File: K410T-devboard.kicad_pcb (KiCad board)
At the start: 2 copper layers, 120 x 120 mm, 31 parts, among them U1 XC7K410T-2FFG900I, U2 MT41K512M8DA

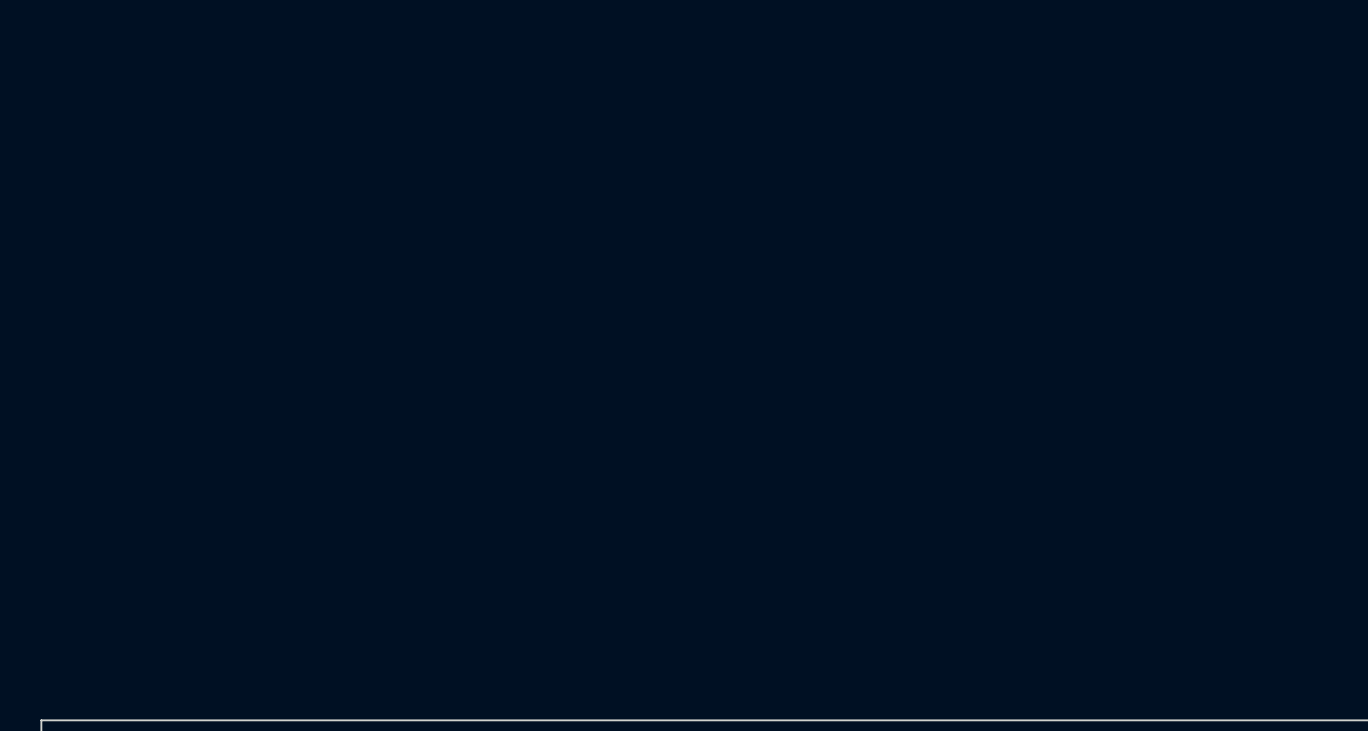
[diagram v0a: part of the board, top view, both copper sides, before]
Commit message: Update project files naming, reorganize hierarchical sheet structure, power supply WIP
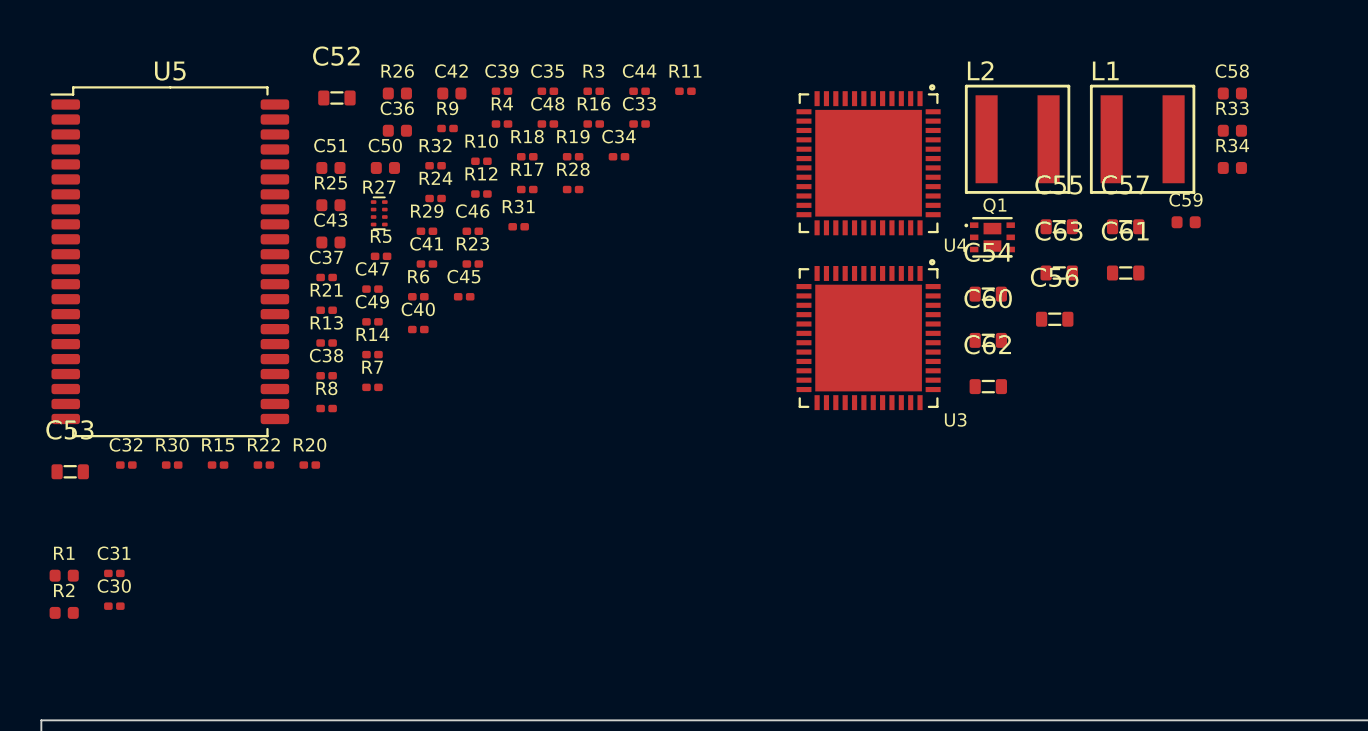
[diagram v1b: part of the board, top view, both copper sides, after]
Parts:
- added C30: C_100n_0201, antmicro-footprints:0201-res, F.Cu at (153.9, 63.9)
- added C31: C_100n_0201, antmicro-footprints:0201-res, F.Cu at (153.9, 62.1)
- added C32: C_100n_0201, antmicro-footprints:0201-res, F.Cu at (154.5, 56.4)
- added C33: C_100n_0201, antmicro-footprints:0201-res, F.Cu at (182.0, 38.1)
- added C34: C_100n_0201, antmicro-footprints:0201-res, F.Cu at (180.9, 39.9)
- added C35: C_100n_0201, antmicro-footprints:0201-res, F.Cu at (177.1, 36.4)
- added C36: C_10u_0402, antmicro-footprints:0402-cap, F.Cu at (169.0, 38.5)
- added C37: C_100n_0201, antmicro-footprints:0201-res, F.Cu at (165.2, 46.3)
- added C38: C_100n_0201, antmicro-footprints:0201-res, F.Cu at (165.2, 51.6)
- added C39: C_100n_0201, antmicro-footprints:0201-res, F.Cu at (174.6, 36.4)
- added C40: C_100n_0201, antmicro-footprints:0201-res, F.Cu at (170.1, 49.1)
- added C41: C_100n_0201, antmicro-footprints:0201-res, F.Cu at (170.6, 45.6)
- added C42: C_10u_0402, antmicro-footprints:0402-cap, F.Cu at (171.9, 36.5)
- added C43: C_10u_0402, antmicro-footprints:0402-cap, F.Cu at (165.5, 44.5)
- added C44: C_100n_0201, antmicro-footprints:0201-res, F.Cu at (182.0, 36.4)
- added C45: C_100n_0201, antmicro-footprints:0201-res, F.Cu at (172.6, 47.4)
- added C46: C_100n_0201, antmicro-footprints:0201-res, F.Cu at (173.1, 43.9)
- added C47: C_100n_0201, antmicro-footprints:0201-res, F.Cu at (167.7, 47.0)
- added C48: C_100n_0201, antmicro-footprints:0201-res, F.Cu at (177.1, 38.1)
- added C49: C_100n_0201, antmicro-footprints:0201-res, F.Cu at (167.7, 48.7)
- added C50: C_4u7_0402, antmicro-footprints:0402-cap, F.Cu at (168.4, 40.5)
- added C51: C_4u7_0402, antmicro-footprints:0402-cap, F.Cu at (165.5, 40.5)
- added C52: C_47u_0603, antmicro-footprints:0603-cap, F.Cu at (165.8, 36.8)
- added C53: C_47u_0603, antmicro-footprints:0603-cap, F.Cu at (151.5, 56.7)
- added C54: C_10u_25V_0603, antmicro-footprints:0603-cap, F.Cu at (200.6, 47.2)
- added C55: C_10u_25V_0603, antmicro-footprints:0603-cap, F.Cu at (204.4, 43.6)
- added C56: C_10u_25V_0603, antmicro-footprints:0603-cap, F.Cu at (204.1, 48.6)
- added C57: C_10u_25V_0603, antmicro-footprints:0603-cap, F.Cu at (207.9, 43.6)
- added C58: C_100n_0402, antmicro-footprints:0402-cap, F.Cu at (213.6, 36.5)
- added C59: C_100n_0402, antmicro-footprints:0402-cap, F.Cu at (211.2, 43.4)
- added C60: C_47u_0603, antmicro-footprints:0603-cap, F.Cu at (200.6, 49.7)
- added C61: C_47u_0603, antmicro-footprints:0603-cap, F.Cu at (207.9, 46.1)
- added C62: C_47u_0603, antmicro-footprints:0603-cap, F.Cu at (200.6, 52.2)
- added C63: C_47u_0603, antmicro-footprints:0603-cap, F.Cu at (204.4, 46.1)
- added L1: XAL5030-122MEC, antmicro-footprints:Coilcraft-XAL5030, F.Cu at (208.8, 39.0)
- added L2: XAL5030-122MEC, antmicro-footprints:Coilcraft-XAL5030, F.Cu at (202.2, 39.0)
- added Q1: SIA906EDJ-T1-GE3, antmicro-footprints:VISHAY_PowerPAK_SC70-6L, F.Cu at (200.8, 44.2)
- added R1: R_80R6_0402, antmicro-footprints:0402-res, F.Cu at (151.2, 62.3)
- added R10: R_40R2_0201, antmicro-footprints:0201-res, F.Cu at (173.5, 40.1)
- added R11: R_40R2_0201, antmicro-footprints:0201-res, F.Cu at (184.4, 36.4)
- added R12: R_40R2_0201, antmicro-footprints:0201-res, F.Cu at (173.5, 41.9)
- added R13: R_40R2_0201, antmicro-footprints:0201-res, F.Cu at (165.2, 49.8)
- added R14: R_40R2_0201, antmicro-footprints:0201-res, F.Cu at (167.7, 50.5)
- added R15: R_40R2_0201, antmicro-footprints:0201-res, F.Cu at (159.4, 56.4)
- added R16: R_40R2_0201, antmicro-footprints:0201-res, F.Cu at (179.5, 38.1)
- added R17: R_40R2_0201, antmicro-footprints:0201-res, F.Cu at (176.0, 41.6)
- added R18: R_40R2_0201, antmicro-footprints:0201-res, F.Cu at (176.0, 39.9)
- added R19: R_40R2_0201, antmicro-footprints:0201-res, F.Cu at (178.4, 39.9)
- added R2: R_80R6_0402, antmicro-footprints:0402-res, F.Cu at (151.2, 64.3)
- added R20: R_40R2_0201, antmicro-footprints:0201-res, F.Cu at (164.3, 56.4)
- added R21: R_40R2_0201, antmicro-footprints:0201-res, F.Cu at (165.2, 48.1)
- added R22: R_40R2_0201, antmicro-footprints:0201-res, F.Cu at (161.9, 56.4)
- added R23: R_100R_0201, antmicro-footprints:0201-res, F.Cu at (173.1, 45.6)
- added R24: R_40R2_0201, antmicro-footprints:0201-res, F.Cu at (171.1, 42.1)
- added R25: R_10k_0402, antmicro-footprints:0402-res, F.Cu at (165.5, 42.5)
- added R26: R_240R_1%_0402, antmicro-footprints:0402-res, F.Cu at (169.0, 36.5)
- added R27: 4x39R_0201_array, antmicro-footprints:EXB18V, F.Cu at (168.1, 42.9)
- added R28: R_40R2_0201, antmicro-footprints:0201-res, F.Cu at (178.4, 41.6)
- added R29: R_40R2_0201, antmicro-footprints:0201-res, F.Cu at (170.6, 43.9)
- added R3: R_40R2_0201, antmicro-footprints:0201-res, F.Cu at (179.5, 36.4)
- added R30: R_40R2_0201, antmicro-footprints:0201-res, F.Cu at (157.0, 56.4)
- added R31: R_40R2_0201, antmicro-footprints:0201-res, F.Cu at (175.5, 43.6)
- added R32: R_40R2_0201, antmicro-footprints:0201-res, F.Cu at (171.1, 40.4)
- added R33: R_22k_0402, antmicro-footprints:0402-res, F.Cu at (213.6, 38.5)
- added R34: R_22k_0402, antmicro-footprints:0402-res, F.Cu at (213.6, 40.5)
- added R4: R_40R2_0201, antmicro-footprints:0201-res, F.Cu at (174.6, 38.1)
- added R5: R_40R2_0201, antmicro-footprints:0201-res, F.Cu at (168.2, 45.2)
- added R6: R_40R2_0201, antmicro-footprints:0201-res, F.Cu at (170.1, 47.4)
- added R7: R_40R2_0201, antmicro-footprints:0201-res, F.Cu at (167.7, 52.2)
- added R8: R_40R2_0201, antmicro-footprints:0201-res, F.Cu at (165.2, 53.3)
- added R9: R_40R2_0201, antmicro-footprints:0201-res, F.Cu at (171.7, 38.4)
- added U3: ADP5054ACPZ-R7, antmicro-footprints:Analog_CP_48_13, F.Cu at (194.2, 49.6)
- added U4: ADP5050ACPZ-R7, antmicro-footprints:Analog_CP_48_13, F.Cu at (194.2, 40.2)
- added U5: AS6C8008-55ZIN, antmicro-footprints:TSOP-II-44_10.16x18.41mm_P0.8mm, F.Cu at (156.9, 45.5)
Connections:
- U1 pad AB7: unconnected-(U1-PadAB7) -> Net-(R2-Pad1)
- U1 pad AC1: unconnected-(U1-PadAC1) -> /FPGA banks 33-34/DDR.A12
- U1 pad AC2: unconnected-(U1-PadAC2) -> /FPGA banks 33-34/DDR.A13
- U1 pad AC4: unconnected-(U1-PadAC4) -> /FPGA banks 33-34/DDR.A10
- U1 pad AC5: unconnected-(U1-PadAC5) -> /FPGA banks 33-34/DDR.A11
- U1 pad AC6: unconnected-(U1-PadAC6) -> /FPGA banks 33-34/DDR_VRN
- U1 pad AC7: unconnected-(U1-PadAC7) -> /FPGA banks 33-34/DDR.A7
- U1 pad AD1: unconnected-(U1-PadAD1) -> /FPGA banks 33-34/DDR.CK_N
- U1 pad AD2: unconnected-(U1-PadAD2) -> /FPGA banks 33-34/DDR.CK_P
- U1 pad AD3: unconnected-(U1-PadAD3) -> /FPGA banks 33-34/DDR.A14
- U1 pad AD4: unconnected-(U1-PadAD4) -> /FPGA banks 33-34/DDR.A15
- U1 pad AD6: unconnected-(U1-PadAD6) -> /FPGA banks 33-34/DDR.A9
- U1 pad AD7: unconnected-(U1-PadAD7) -> /FPGA banks 33-34/+0.676_VTT
- U1 pad AE1: unconnected-(U1-PadAE1) -> /FPGA banks 33-34/DDR.A4
- U1 pad AE3: unconnected-(U1-PadAE3) -> /FPGA banks 33-34/DDR.BA2
- U1 pad AE4: unconnected-(U1-PadAE4) -> /FPGA banks 33-34/DDR.A0
- U1 pad AE5: unconnected-(U1-PadAE5) -> /FPGA banks 33-34/DDR.BA1
- U1 pad AE6: unconnected-(U1-PadAE6) -> /FPGA banks 33-34/DDR.A8
- U1 pad AF1: unconnected-(U1-PadAF1) -> /FPGA banks 33-34/DDR.A3
- U1 pad AF2: unconnected-(U1-PadAF2) -> /FPGA banks 33-34/DDR.A5
- U1 pad AF3: unconnected-(U1-PadAF3) -> /FPGA banks 33-34/DDR.A6
- U1 pad AF5: unconnected-(U1-PadAF5) -> /FPGA banks 33-34/DDR.BA0
- U1 pad AF6: unconnected-(U1-PadAF6) -> /FPGA banks 33-34/DDR.~{CAS}
- U1 pad AF7: unconnected-(U1-PadAF7) -> /FPGA banks 33-34/DDR.DQ0
- U1 pad AF8: unconnected-(U1-PadAF8) -> /FPGA banks 33-34/DDR.DM
- U1 pad AG2: unconnected-(U1-PadAG2) -> /FPGA banks 33-34/DDR.~{WE}
- U1 pad AG3: unconnected-(U1-PadAG3) -> /FPGA banks 33-34/DDR.A1
- U1 pad AG4: unconnected-(U1-PadAG4) -> /FPGA banks 33-34/DDR.A2
- U1 pad AG5: unconnected-(U1-PadAG5) -> /FPGA banks 33-34/DDR.~{RAS}
- U1 pad AG7: unconnected-(U1-PadAG7) -> /FPGA banks 33-34/DDR.DQ1
- U1 pad AG8: unconnected-(U1-PadAG8) -> /FPGA banks 33-34/+0.676_VTT
- U1 pad AH1: unconnected-(U1-PadAH1) -> /FPGA banks 33-34/DDR.~{CS}
- U1 pad AH2: unconnected-(U1-PadAH2) -> /FPGA banks 33-34/DDR.CKE
- U1 pad AH4: unconnected-(U1-PadAH4) -> /FPGA banks 33-34/DDR.~{RESET}
- U1 pad AH7: unconnected-(U1-PadAH7) -> /FPGA banks 33-34/DDR.DQS_P
- U1 pad AJ2: unconnected-(U1-PadAJ2) -> /FPGA banks 33-34/DDR.ODT
- U1 pad AJ6: unconnected-(U1-PadAJ6) -> /FPGA banks 33-34/DDR.DQ2
- U1 pad AJ7: unconnected-(U1-PadAJ7) -> /FPGA banks 33-34/DDR.DQS_N
- U1 pad AJ8: unconnected-(U1-PadAJ8) -> /FPGA banks 33-34/DDR.DQ4
- U1 pad AK4: unconnected-(U1-PadAK4) -> /FPGA banks 33-34/DDR.DQ7
- U1 pad AK5: unconnected-(U1-PadAK5) -> /FPGA banks 33-34/DDR.DQ6
- U1 pad AK6: unconnected-(U1-PadAK6) -> /FPGA banks 33-34/DDR.DQ3
- U1 pad AK8: unconnected-(U1-PadAK8) -> /FPGA banks 33-34/DDR.DQ5
- U1 pad P26: unconnected-(U1-PadP26) -> /FPGA banks 12-15/SRAM.~{OE}
- U1 pad P27: unconnected-(U1-PadP27) -> /FPGA banks 12-15/SRAM.A5
- U1 pad P28: unconnected-(U1-PadP28) -> /FPGA banks 12-15/SRAM.A6
- U1 pad P29: unconnected-(U1-PadP29) -> /FPGA banks 12-15/SRAM.DQ3
- U1 pad R26: unconnected-(U1-PadR26) -> /FPGA banks 12-15/SRAM.A8
- U1 pad R28: unconnected-(U1-PadR28) -> /FPGA banks 12-15/SRAM.DQ6
- U1 pad R29: unconnected-(U1-PadR29) -> /FPGA banks 12-15/SRAM.DQ7
- U1 pad R30: unconnected-(U1-PadR30) -> /FPGA banks 12-15/SRAM.A9
- U1 pad T25: unconnected-(U1-PadT25) -> /FPGA banks 12-15/SRAM.A2
- U1 pad T26: unconnected-(U1-PadT26) -> /FPGA banks 12-15/SRAM.A3
- U1 pad T27: unconnected-(U1-PadT27) -> /FPGA banks 12-15/SRAM.A13
- U1 pad T28: unconnected-(U1-PadT28) -> /FPGA banks 12-15/SRAM.DQ5
- U1 pad T30: unconnected-(U1-PadT30) -> /FPGA banks 12-15/SRAM.A15
- U1 pad U20: unconnected-(U1-PadU20) -> /FPGA banks 12-15/SRAM.DQ4
- U1 pad U22: unconnected-(U1-PadU22) -> /FPGA banks 12-15/SRAM.CE2
- U1 pad U23: unconnected-(U1-PadU23) -> /FPGA banks 12-15/SRAM.A14
- U1 pad U25: unconnected-(U1-PadU25) -> /FPGA banks 12-15/SRAM.A11
- U1 pad U27: unconnected-(U1-PadU27) -> /FPGA banks 12-15/SRAM.A10
- U1 pad U28: unconnected-(U1-PadU28) -> /FPGA banks 12-15/SRAM.A0
- U1 pad V19: unconnected-(U1-PadV19) -> /FPGA banks 12-15/SRAM.A12
- U1 pad V20: unconnected-(U1-PadV20) -> /FPGA banks 12-15/SRAM.A4
- U1 pad V21: unconnected-(U1-PadV21) -> /FPGA banks 12-15/SRAM.DQ0
- U1 pad V24: unconnected-(U1-PadV24) -> /FPGA banks 12-15/SRAM.A7
- U1 pad V25: unconnected-(U1-PadV25) -> /FPGA banks 12-15/SRAM.A18
- U1 pad V27: unconnected-(U1-PadV27) -> /FPGA banks 12-15/SRAM.~{CE}
- U1 pad V29: unconnected-(U1-PadV29) -> /FPGA banks 12-15/SRAM.A1
- U1 pad V30: unconnected-(U1-PadV30) -> /FPGA banks 12-15/SRAM.DQ1
- U1 pad W21: unconnected-(U1-PadW21) -> /FPGA banks 12-15/SRAM.DQ2
- U1 pad W22: unconnected-(U1-PadW22) -> /FPGA banks 12-15/SRAM.~{WE}
- U1 pad W23: unconnected-(U1-PadW23) -> /FPGA banks 12-15/SRAM.A16
- U1 pad W24: unconnected-(U1-PadW24) -> /FPGA banks 12-15/SRAM.A17
- U1 pad W26: unconnected-(U1-PadW26) -> /FPGA banks 12-15/SRAM.A19
- U2 pad A1: VSS -> GND
- U2 pad A2: VDD -> +1V35
- U2 pad A8: VSS -> GND
- U2 pad A9: VDD -> +1V35
- U2 pad B1: VSS -> GND
- U2 pad B2: VSSQ -> GND
- U2 pad B3: unconnected-(U2-PadB3) -> /FPGA banks 33-34/DDR.DQ0
- U2 pad B7: unconnected-(U2-PadB7) -> /FPGA banks 33-34/DDR.DM
- U2 pad B8: VSSQ -> GND
- U2 pad B9: VDDQ -> +1V35
- U2 pad C1: VDDQ -> +1V35
- U2 pad C2: unconnected-(U2-PadC2) -> /FPGA banks 33-34/DDR.DQ2
- U2 pad C3: unconnected-(U2-PadC3) -> /FPGA banks 33-34/DDR.DQS_P
- U2 pad C7: unconnected-(U2-PadC7) -> /FPGA banks 33-34/DDR.DQ1
- U2 pad C8: unconnected-(U2-PadC8) -> /FPGA banks 33-34/DDR.DQ3
- U2 pad C9: VSSQ -> GND
- U2 pad D1: VSSQ -> GND
- U2 pad D2: unconnected-(U2-PadD2) -> /FPGA banks 33-34/DDR.DQ6
- U2 pad D3: unconnected-(U2-PadD3) -> /FPGA banks 33-34/DDR.DQS_N
- U2 pad D7: VDD -> +1V35
- U2 pad D8: VSS -> GND
- U2 pad D9: VSSQ -> GND
- U2 pad E1: unconnected-(U2-PadE1) -> /RAM/+0.676_VREF
- U2 pad E2: VDDQ -> +1V35
- U2 pad E3: unconnected-(U2-PadE3) -> /FPGA banks 33-34/DDR.DQ4
- U2 pad E7: unconnected-(U2-PadE7) -> /FPGA banks 33-34/DDR.DQ7
- U2 pad E8: unconnected-(U2-PadE8) -> /FPGA banks 33-34/DDR.DQ5
- U2 pad E9: VDDQ -> +1V35
- U2 pad F2: VSS -> GND
- U2 pad F3: unconnected-(U2-PadF3) -> /FPGA banks 33-34/DDR.~{RAS}
- U2 pad F7: unconnected-(U2-PadF7) -> /FPGA banks 33-34/DDR.CK_P
- U2 pad F8: VSS -> GND
- U2 pad G1: unconnected-(U2-PadG1) -> /FPGA banks 33-34/DDR.ODT
- U2 pad G2: VDD -> +1V35
- U2 pad G3: unconnected-(U2-PadG3) -> /FPGA banks 33-34/DDR.~{CAS}
- U2 pad G7: unconnected-(U2-PadG7) -> /FPGA banks 33-34/DDR.CK_N
- U2 pad G8: VDD -> +1V35
- U2 pad G9: unconnected-(U2-PadG9) -> /FPGA banks 33-34/DDR.CKE
- U2 pad H2: unconnected-(U2-PadH2) -> /FPGA banks 33-34/DDR.~{CS}
- U2 pad H3: unconnected-(U2-PadH3) -> /FPGA banks 33-34/DDR.~{WE}
- U2 pad H7: unconnected-(U2-PadH7) -> /FPGA banks 33-34/DDR.A10
- U2 pad H8: unconnected-(U2-PadH8) -> /RAM/DDR_ZQ
- U2 pad J1: VSS -> GND
- U2 pad J2: unconnected-(U2-PadJ2) -> /FPGA banks 33-34/DDR.BA0
- U2 pad J3: unconnected-(U2-PadJ3) -> /FPGA banks 33-34/DDR.BA2
- U2 pad J7: unconnected-(U2-PadJ7) -> /FPGA banks 33-34/DDR.A15
- U2 pad J8: unconnected-(U2-PadJ8) -> /RAM/+0.676_VREF
- U2 pad J9: VSS -> GND
- U2 pad K1: VDD -> +1V35
- U2 pad K2: unconnected-(U2-PadK2) -> /FPGA banks 33-34/DDR.A3
- U2 pad K3: unconnected-(U2-PadK3) -> /FPGA banks 33-34/DDR.A0
- U2 pad K7: unconnected-(U2-PadK7) -> /FPGA banks 33-34/DDR.A12
- U2 pad K8: unconnected-(U2-PadK8) -> /FPGA banks 33-34/DDR.BA1
- U2 pad K9: VDD -> +1V35
- U2 pad L1: VSS -> GND
- U2 pad L2: unconnected-(U2-PadL2) -> /FPGA banks 33-34/DDR.A5
- U2 pad L3: unconnected-(U2-PadL3) -> /FPGA banks 33-34/DDR.A2
- U2 pad L7: unconnected-(U2-PadL7) -> /FPGA banks 33-34/DDR.A1
- U2 pad L8: unconnected-(U2-PadL8) -> /FPGA banks 33-34/DDR.A4
- U2 pad L9: VSS -> GND
- U2 pad M1: VDD -> +1V35
- U2 pad M2: unconnected-(U2-PadM2) -> /FPGA banks 33-34/DDR.A7
- U2 pad M3: unconnected-(U2-PadM3) -> /FPGA banks 33-34/DDR.A9
- U2 pad M7: unconnected-(U2-PadM7) -> /FPGA banks 33-34/DDR.A11
- U2 pad M8: unconnected-(U2-PadM8) -> /FPGA banks 33-34/DDR.A6
- U2 pad M9: VDD -> +1V35
- U2 pad N1: VSS -> GND
- U2 pad N2: unconnected-(U2-PadN2) -> /FPGA banks 33-34/DDR.~{RESET}
- U2 pad N3: unconnected-(U2-PadN3) -> /FPGA banks 33-34/DDR.A13
- U2 pad N7: unconnected-(U2-PadN7) -> /FPGA banks 33-34/DDR.A14
- U2 pad N8: unconnected-(U2-PadN8) -> /FPGA banks 33-34/DDR.A8
- U2 pad N9: VSS -> GND
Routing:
- net GND: track 122.3 -> 131.9 mm, vias 173 -> 190
- net +1V35: track 0.00 -> 7.35 mm, vias 0 -> 13
- net VSS: track 6.79 -> 0.00 mm, vias 12 -> 0
- net VDD: track 5.09 -> 0.00 mm, vias 9 -> 0
- net VSSQ: track 2.83 -> 0.00 mm, vias 5 -> 0
- net VDDQ: track 2.26 -> 0.00 mm, vias 4 -> 0
- net /FPGA banks 33-34/+0.676_VTT: track 0.00 -> 1.41 mm, vias 0 -> 2
- net /FPGA banks 33-34/DDR.~{WE}: track 0.00 -> 1.27 mm, vias 0 -> 2
- net /FPGA banks 33-34/DDR.~{RESET}: track 0.00 -> 1.27 mm, vias 0 -> 2
- net /FPGA banks 33-34/DDR.~{RAS}: track 0.00 -> 1.27 mm, vias 0 -> 2
- net /FPGA banks 33-34/DDR.~{CS}: track 0.00 -> 1.27 mm, vias 0 -> 2
- net /FPGA banks 33-34/DDR.~{CAS}: track 0.00 -> 1.27 mm, vias 0 -> 2
- net /FPGA banks 33-34/DDR.ODT: track 0.00 -> 1.27 mm, vias 0 -> 2
- net /FPGA banks 33-34/DDR.DQ7: track 0.00 -> 1.27 mm, vias 0 -> 2
- net /FPGA banks 33-34/DDR.DQ5: track 0.00 -> 1.27 mm, vias 0 -> 2
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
